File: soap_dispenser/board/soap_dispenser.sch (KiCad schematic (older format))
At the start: 43 parts, among them M1 Motor_DC, Q1 PMOS, Q11 NMOS, Q3 PMOS, Q4 NMOS, Q5 NMOS, SW1 SW_SPDT, SW8 SW_Push, U1 ATtiny48-AU

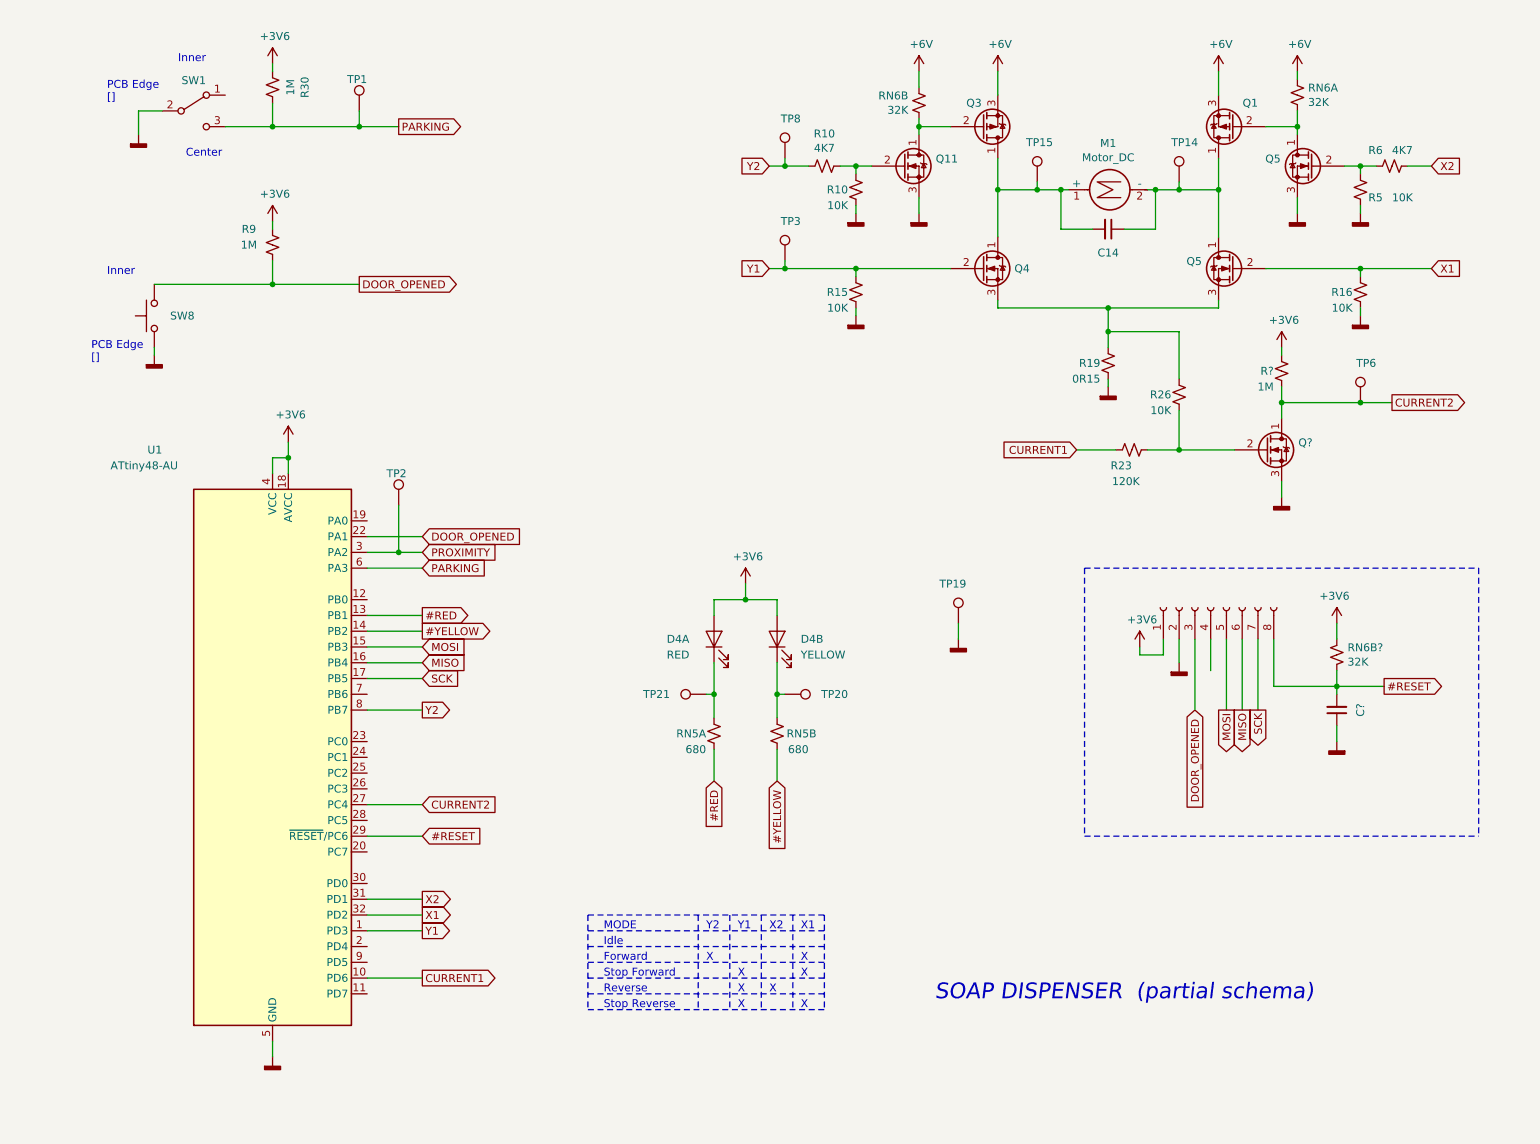
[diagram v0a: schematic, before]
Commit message: Updated schema and capture files.
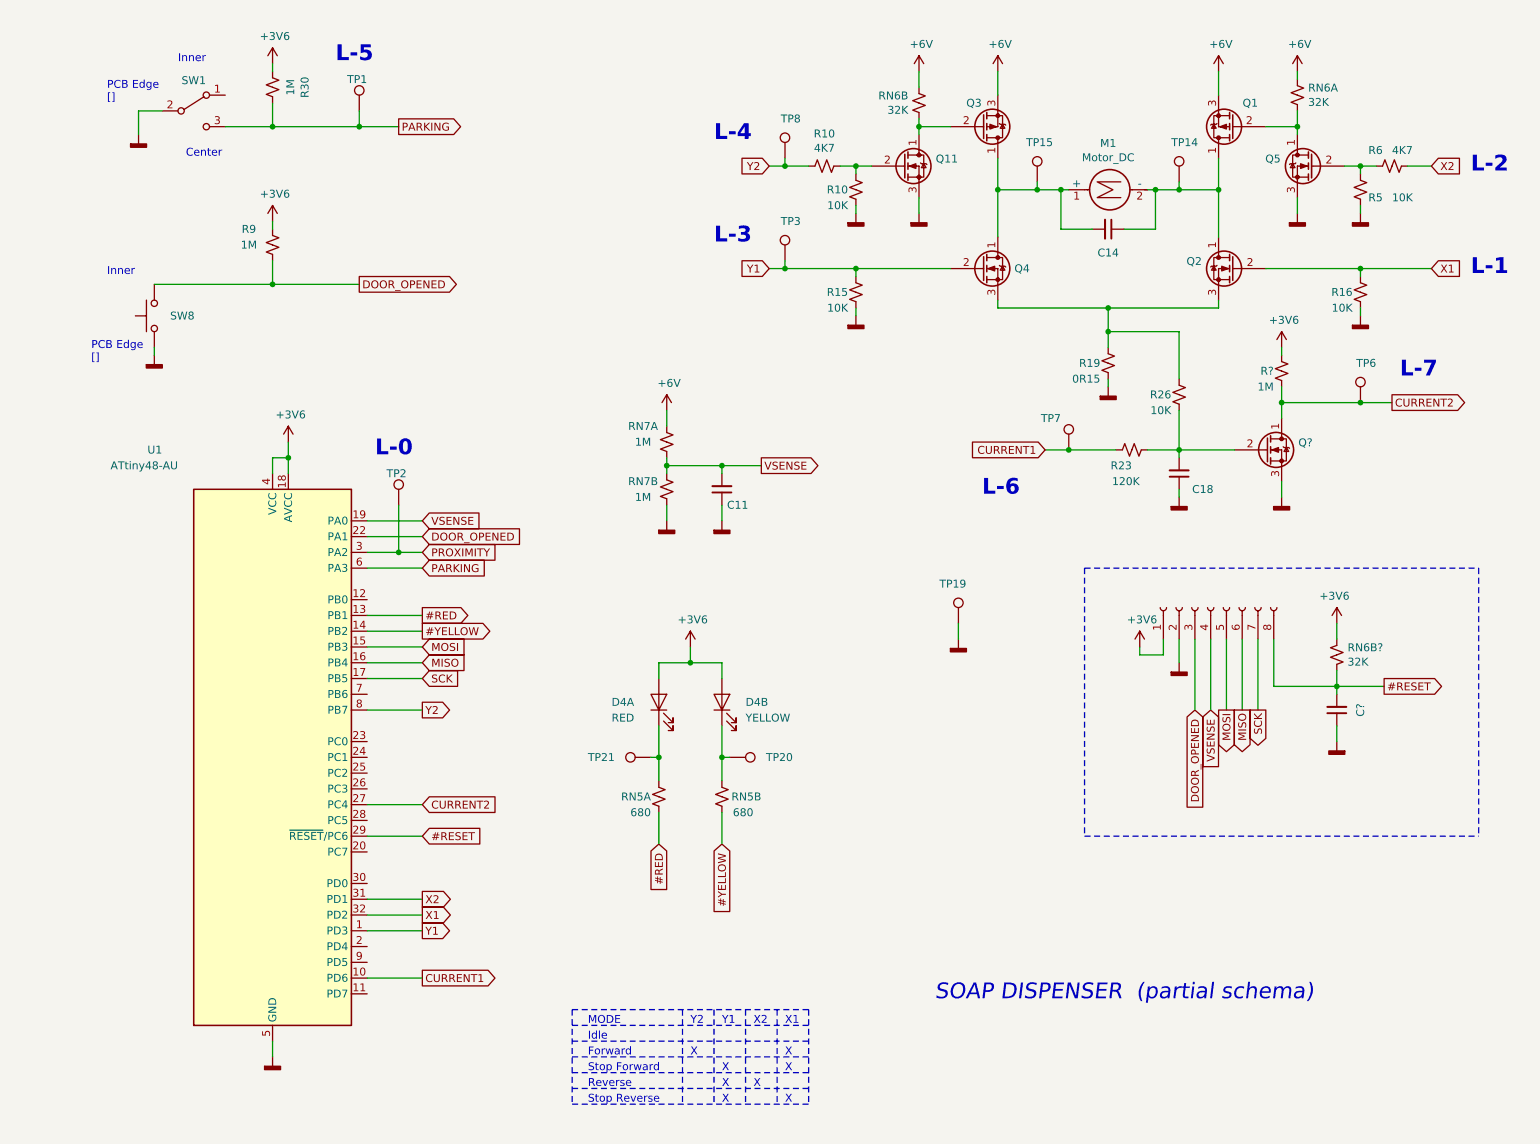
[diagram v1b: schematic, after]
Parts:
- added C11, C18: C_Small, symbol Device:C_Small
- added RN7A, RN7B: 1M, symbol Device:R_Small_US
- added TP7: TestPoint, symbol Connector:TestPoint
- renumbered Q5 to Q2
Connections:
- net +6V: now also RN7A.1
- net CURRENT1: now also TP7.1
- net GNDD: now also C11.1, C18.1, RN7B.2
- net VSENSE: now reaches U1.19 (PA0)
- net VSENSE: now also J?.4 (Pin_4), C11.2, RN7A.2, RN7B.1
- net at Q?.2 (G), R23.2, R26.1: now also C18.2
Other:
- note added: "L-0"
- note added: "L-1"
- note added: "L-2"
- note added: "L-3"
- note added: "L-4"
- note added: "L-5"
- note added: "L-6"
- note added: "L-7"
- moved on the sheet: D4A, D4B, RN5A, RN5B, TP20, TP21

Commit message: Minor schema cleanup
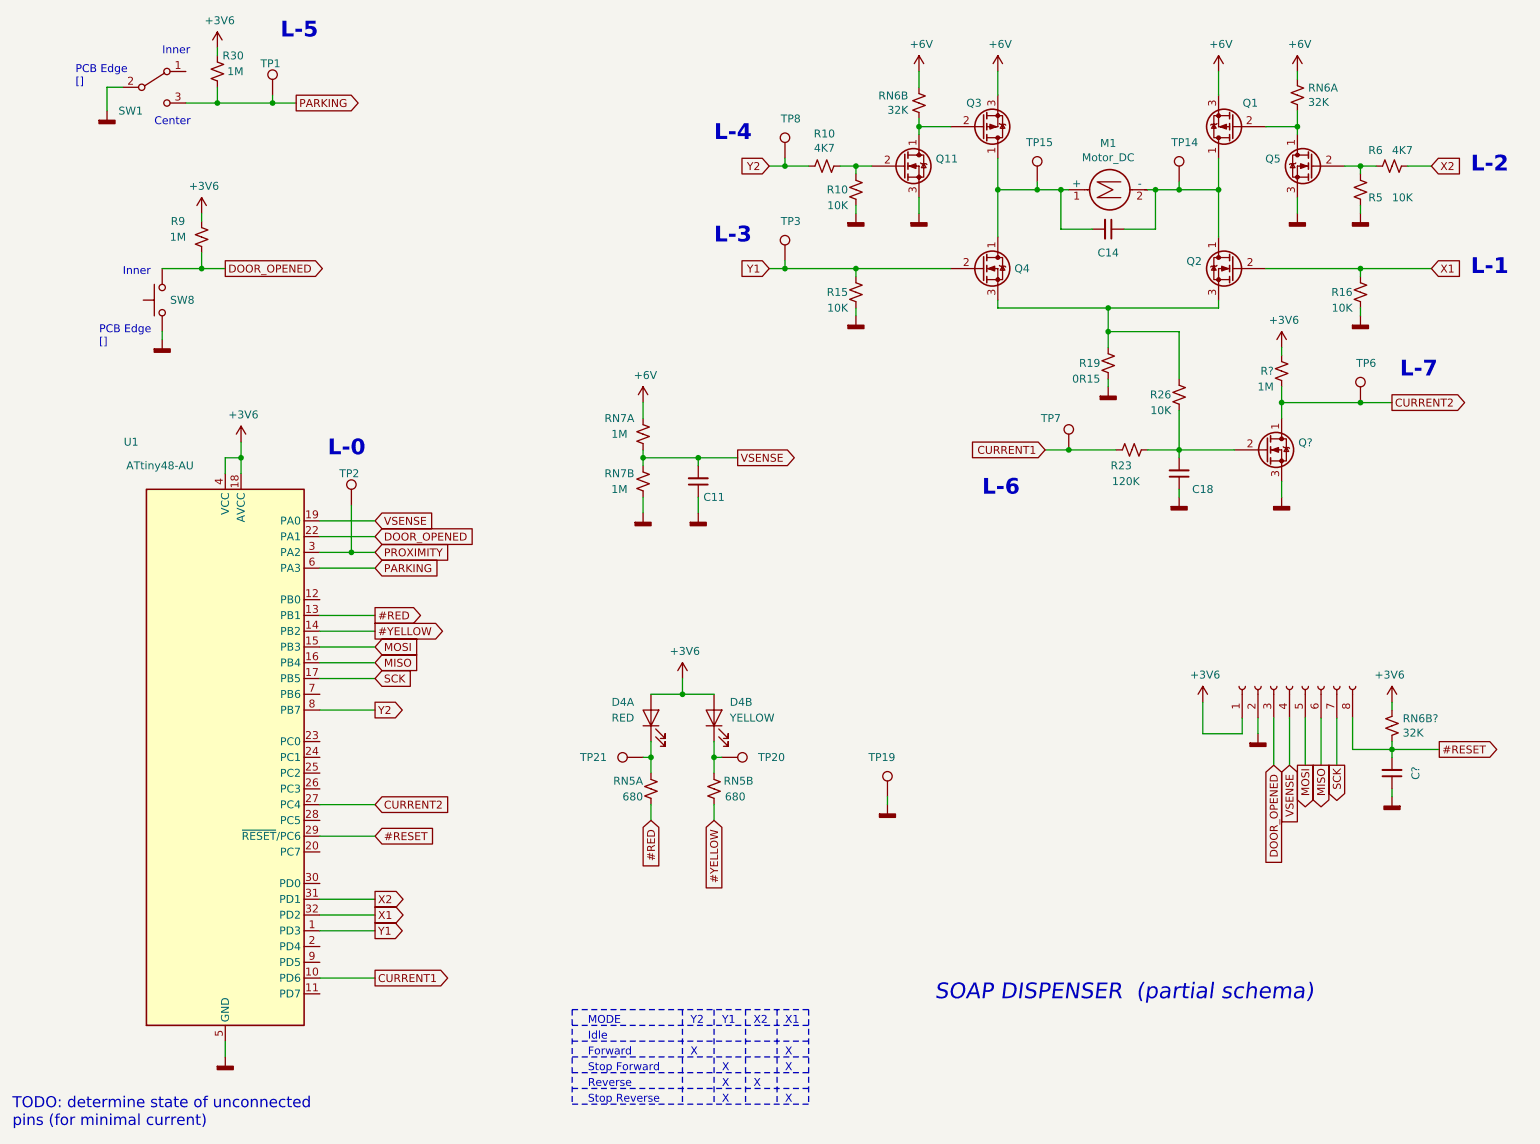
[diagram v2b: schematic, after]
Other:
- note added: "TODO: determine state of unconnected\npins (for minimal current)"
- moved on the sheet: C11, C?, D4A, D4B, R30, R9, RN5A, RN5B, RN6B?, RN7A, RN7B, SW1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
